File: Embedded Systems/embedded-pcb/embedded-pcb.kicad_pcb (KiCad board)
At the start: 2 copper layers, 19 parts, among them J1 Servos, U1 LM324

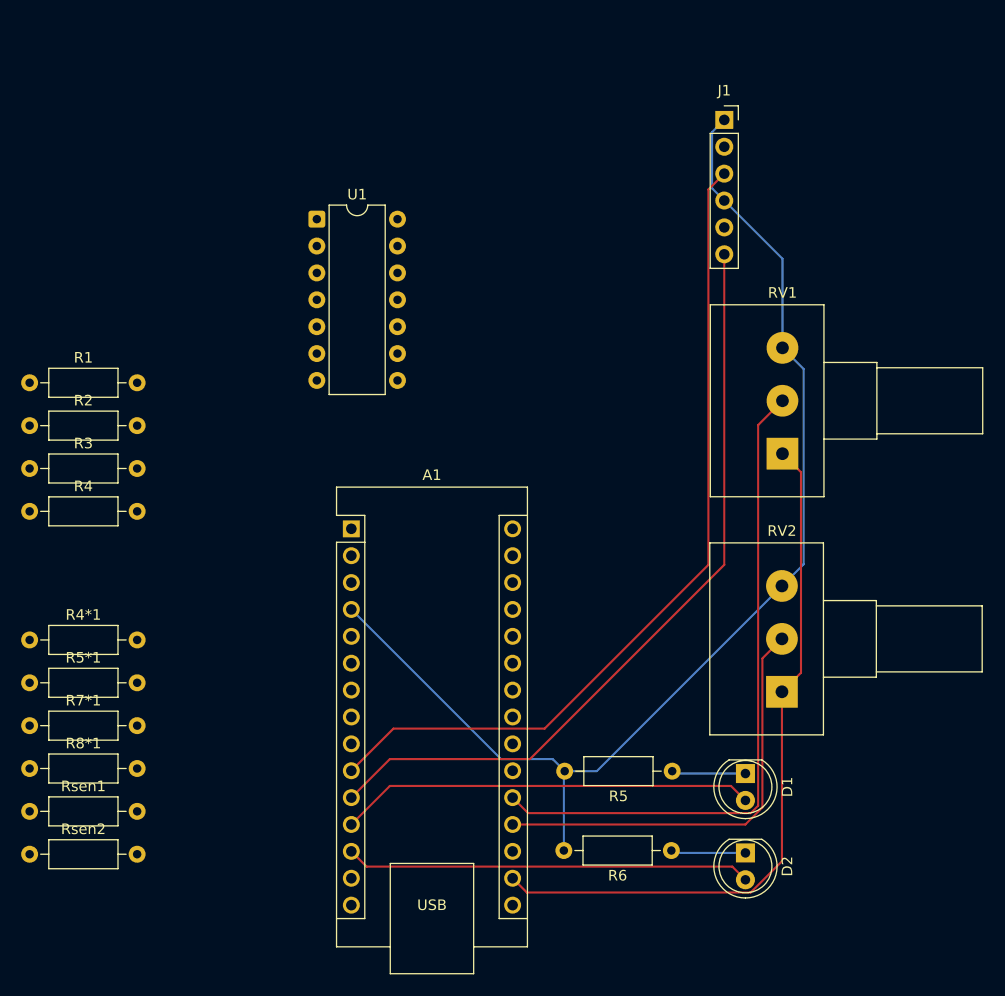
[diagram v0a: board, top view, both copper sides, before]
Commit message: feat: updated schematic
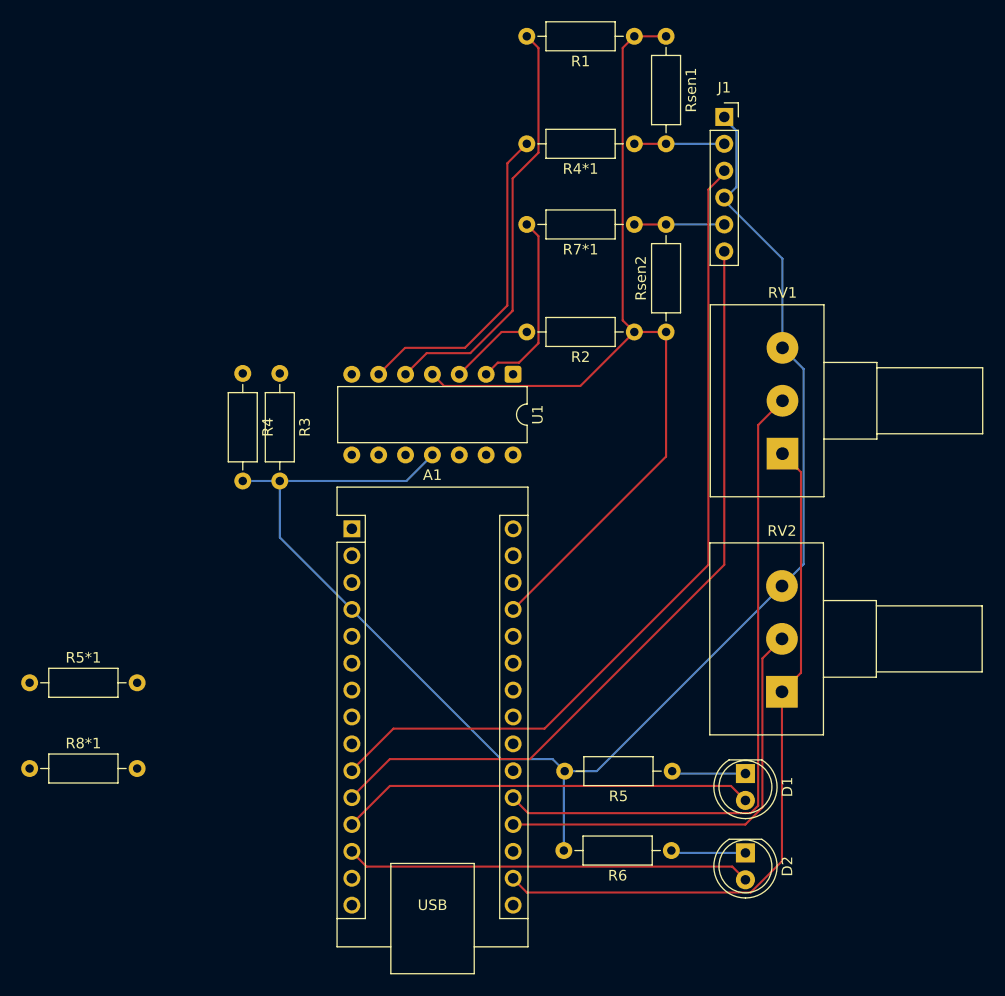
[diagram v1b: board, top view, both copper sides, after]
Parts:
- moved Rsen1 94.8 mm to (169.0, 22.6), turned to -90 degrees
- moved Rsen2 77.8 mm to (169.0, 50.5), turned to 90 degrees
- moved R7*1 74.2 mm to (166.0, 40.3), turned to 180 degrees
- moved R4*1 73.9 mm to (166.0, 32.7), turned to 180 degrees
- moved R1 65.9 mm to (166.0, 22.6), turned to 180 degrees
- moved R2 57.8 mm to (166.0, 50.5), turned to 180 degrees
- moved R3 25.3 mm to (132.5, 54.4), turned to -90 degrees
- moved R4 24.0 mm to (129.0, 54.4), turned to -90 degrees
- moved U1 23.6 mm to (154.5, 54.5), turned to -90 degrees
- moved J1 0.28 mm to (174.5, 30.2)
- moved A1 0.05 mm to (139.3, 69.1)
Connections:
- R1 pad 2: Net-(U1A-+) -> Net-(U1B-+)
- R2 pad 2: Net-(U1B-+) -> Net-(U1A-+)
- R3 pad 1: Net-(U1A-+) -> Net-(U1B-+)
- R4 pad 1: Net-(U1B-+) -> Net-(U1A-+)
- R4*1 pad 2: Net-(U1A--) -> Net-(U1B--)
- R5*1 pad 1: Net-(U1A--) -> Net-(U1B--)
- R7*1 pad 2: Net-(U1B--) -> Net-(U1A--)
- R8*1 pad 1: Net-(U1B--) -> Net-(U1A--)
- U1 pad 1: Net-(A1-A3) -> Net-(A1-A2)
- U1 pad 7: Net-(A1-A2) -> Net-(A1-A3)
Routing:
- net Net-(A1-+5V): track 0.00 -> 88.7 mm
- net Net-(U1B-+): track 0.00 -> 40.0 mm
- net /GND: track 110.8 -> 144.7 mm
- net Net-(U1B--): track 0.00 -> 30.9 mm
- net Net-(U1A--): track 0.00 -> 17.8 mm
- net /Vcc: track 0.00 -> 17.0 mm
- net Net-(U1A-+): track 0.00 -> 8.04 mm
